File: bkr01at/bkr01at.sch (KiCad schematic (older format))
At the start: 41 parts, among them J1 Conn_02x03_Odd_Even, J2 Conn_01x02_Female, SW1 SW_Push, SW2 SW_Push, SW3 SW_Push, U1 nRF52832-QFAB, Y1 32.768kHz, Y2 32MHz

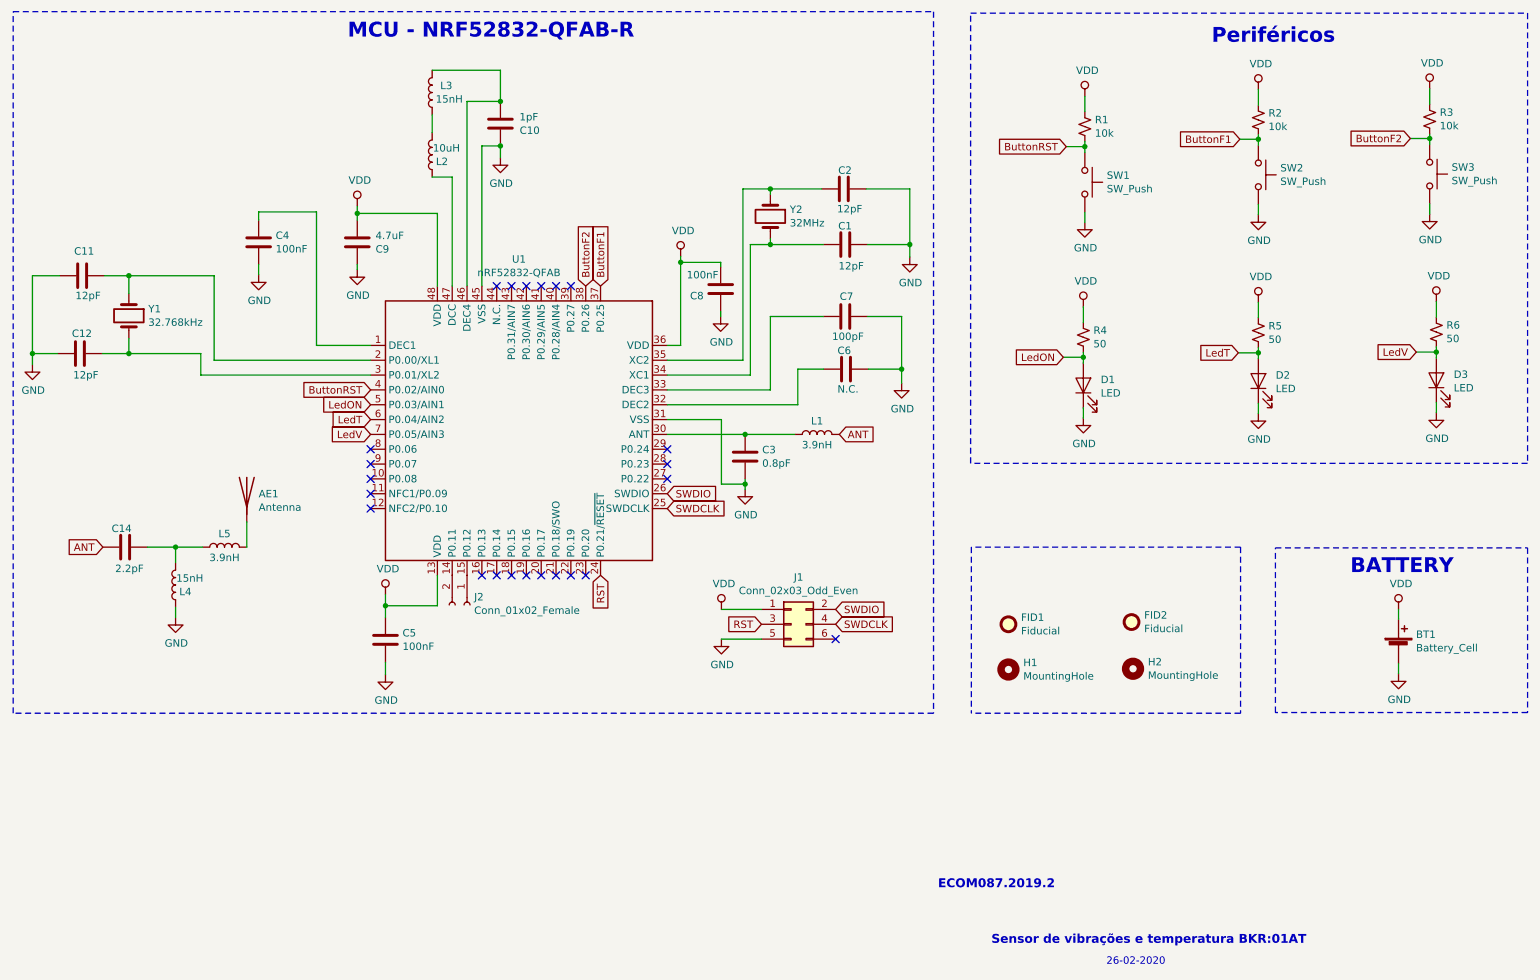
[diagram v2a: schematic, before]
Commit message: Esquemático ok. PCB is loading.
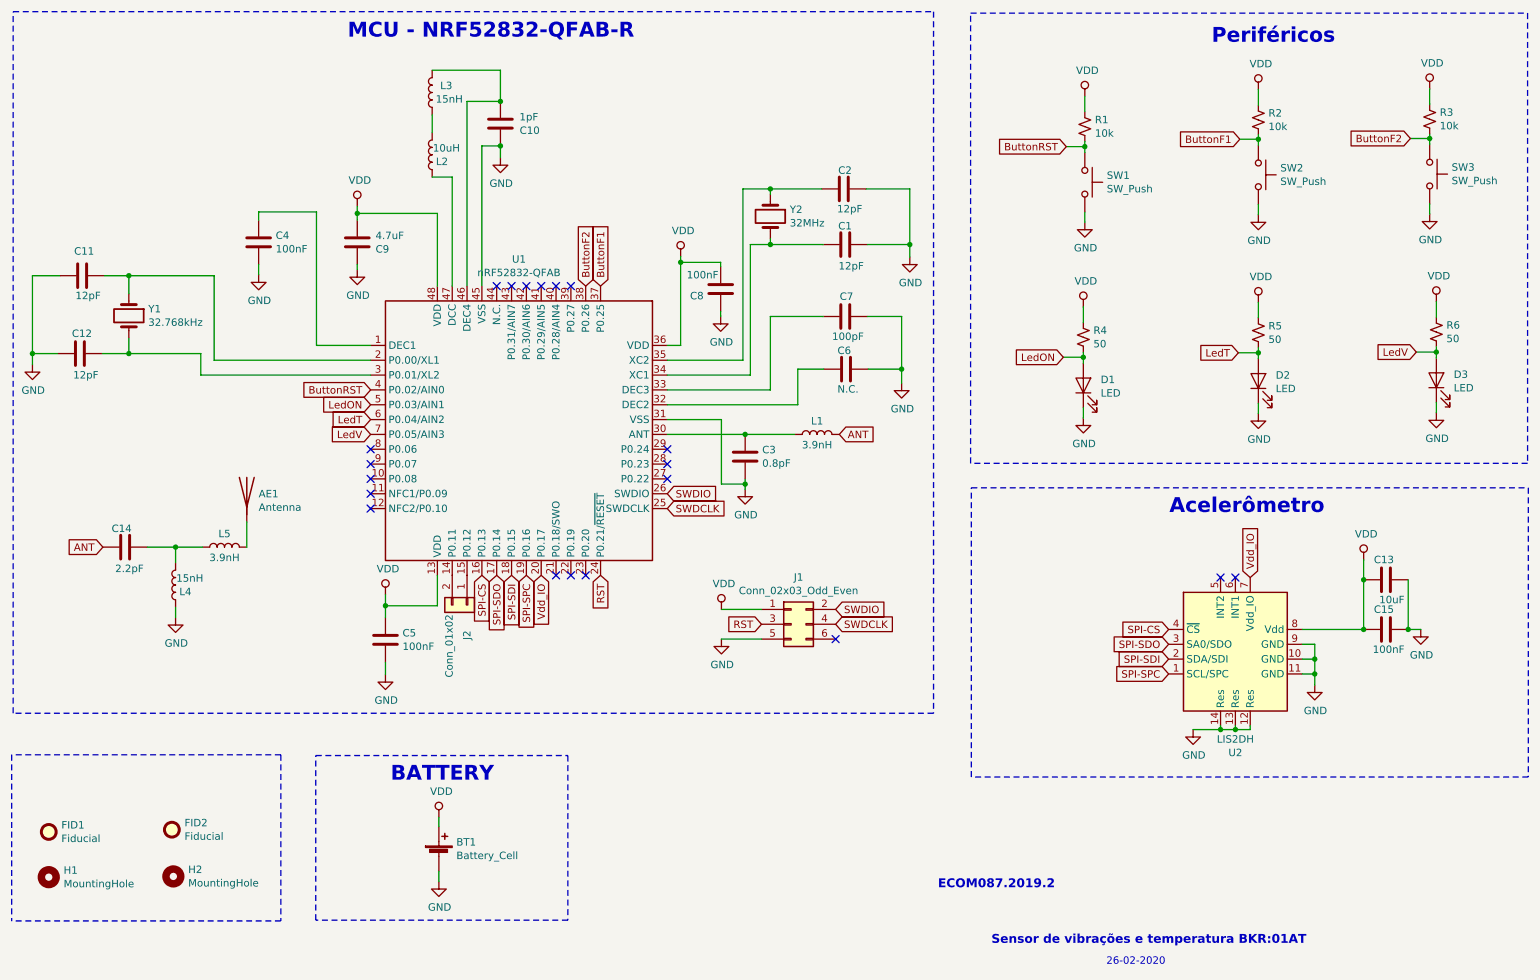
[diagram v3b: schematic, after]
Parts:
- removed J2: Conn_01x02_Female, Connector:Banana_Jack_2Pin, symbol Connector:Conn_01x02_Female
- added C13: 10uF, Capacitor_SMD:C_0402_1005Metric, symbol Device:C
- added C15: 100nF, Capacitor_SMD:C_0402_1005Metric, symbol Device:C
- added J2: Conn_01x02, Connector_Wire:SolderWirePad_1x02_P3.81mm_Drill0.8mm, symbol Connector_Generic:Conn_01x02
- added U2: LIS2DH, Package_LGA:LGA-14_2x2mm_P0.35mm_LayoutBorder3x4y, symbol sensor_motion:LIS2DH
- BT1: footprint Battery:Battery_CR1225 -> Battery:Battery_Panasonic_CR2032-VS1N_Vertical_CircularHoles
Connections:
- net GND: now also C13.2, C15.2, U2.10 (GND), U2.11 (GND), U2.12 (Res), U2.13 (Res), U2.14 (Res), U2.9 (GND)
- net VDD: now also C13.1, C15.1, U2.8 (Vdd)
- net at U1.14 (P0.11): now also J2.2 (Pin_2)
- net at U1.15 (P0.12): now also J2.1 (Pin_1)
- net SPI-CS: now reaches U1.16 (P0.13)
- net SPI-CS: now also U2.4 (~CS)
- net SPI-SDO: now reaches U1.17 (P0.14)
- net SPI-SDO: now also U2.3 (SA0/SDO)
- net SPI-SDI: now reaches U1.18 (P0.15)
- net SPI-SDI: now also U2.2 (SDA/SDI)
- net SPI-SPC: now reaches U1.19 (P0.16)
- net SPI-SPC: now also U2.1 (SCL/SPC)
- net Vdd_IO: now reaches U1.20 (P0.17)
- net Vdd_IO: now also U2.7 (Vdd_IO)
- no-connect marks 23 -> 20
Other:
- note added: "Acelerômetro"
- moved on the sheet: BT1, FID1, FID2, H1, H2
